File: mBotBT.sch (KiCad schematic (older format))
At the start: 6 parts, among them P101 CONN_01X04, P102 CONN_01X03, U101 LM1084IT-3.3/NOPB, U102 XBEE

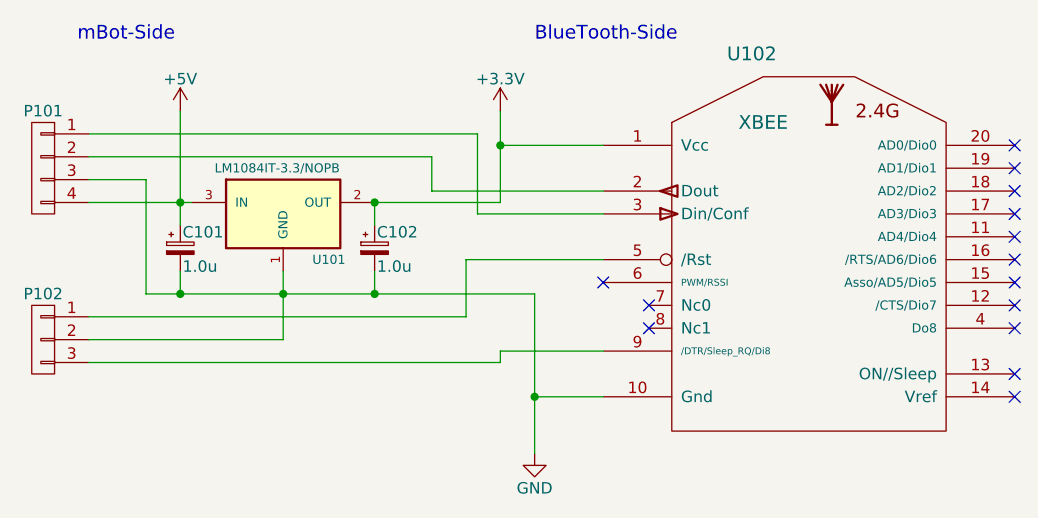
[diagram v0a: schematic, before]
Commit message: Bugfix
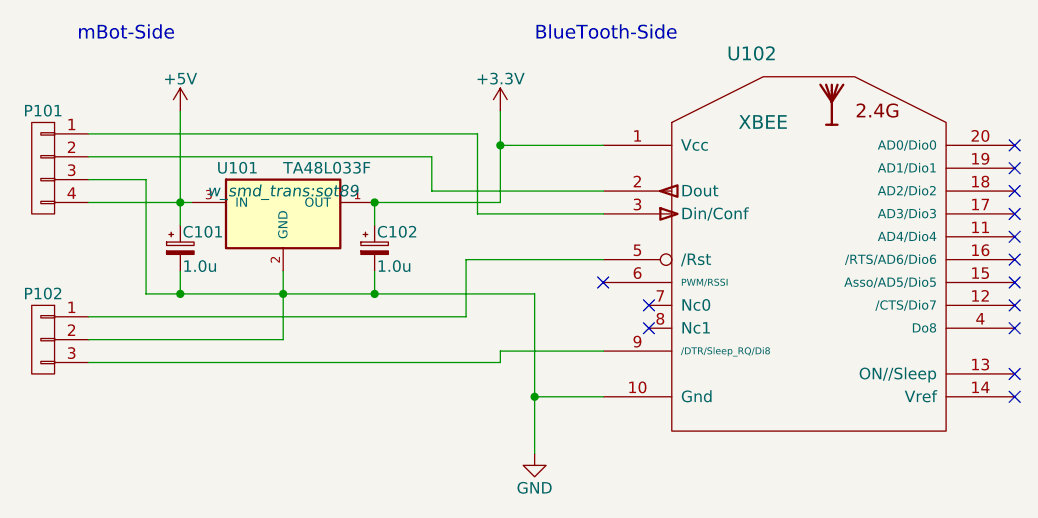
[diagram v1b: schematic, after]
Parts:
- removed U101: LM1084IT-3.3/NOPB, w_smd_trans:sot89, symbol LM1084IT-3.3/NOPB
- added U101: TA48L033F, w_smd_trans:sot89, symbol MC78L08ACH
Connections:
- net +3V3: now also U101.1 (OUT)
- net +5V: now also U101.3 (IN)
- net GND: now also U101.2 (GND)
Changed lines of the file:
@@
 BlueTooth-Side
-$Comp
-L LM1084IT-3.3/NOPB U101
-U 1 1 56B5416D
-P 4700 2500
-F 0 "U101" H 4900 2300 40  0000 C CNN
-F 1 "LM1084IT-3.3/NOPB" H 4400 2700 40  0000 L CNN
-F 2 "w_smd_trans:sot89" H 4700 2600 30  0001 C CIN
-F 3 "" H 4700 2500 60  0000 C CNN
-	1    4700 2500
-	1    0    0    -1
-$EndComp
 $Comp
 L CP_Small C101
@@
 	1    0    0    -1
 $EndComp
+NoConn ~ 6300 3000
+NoConn ~ 6300 2900
+NoConn ~ 6100 2800
+NoConn ~ 7900 2200
+NoConn ~ 7900 2300
+NoConn ~ 7900 2400
+NoConn ~ 7900 2500
+NoConn ~ 7900 2600
+NoConn ~ 7900 2700
+NoConn ~ 7900 2800
+NoConn ~ 7900 2900
+NoConn ~ 7900 3000
+NoConn ~ 7900 3200
+NoConn ~ 7900 3300
 Wire Wire Line
 	3850 2450 4300 2450
@@
 	5350 2250 3850 2250
 Wire Wire Line
-	5650 2450 5100 2450
-Wire Wire Line
-	5650 2050 5650 2450
+	5650 2450 5650 2050
 Wire Wire Line
 	5650 2200 6100 2200
@@
 Connection ~ 4700 2850
 Wire Wire Line
-	5100 2450 5100 2550
-Wire Wire Line
 	4250 2750 4250 2850
 Connection ~ 4250 2850
@@
 	4250 2050 4250 2550
 Connection ~ 4250 2450
-Connection ~ 5100 2450
 Wire Wire Line
 	4700 3050 3850 3050
@@
 Connection ~ 5650 2200
 Connection ~ 5800 3300
-NoConn ~ 6300 3000
-NoConn ~ 6300 2900
-NoConn ~ 6100 2800
-NoConn ~ 7900 2200
-NoConn ~ 7900 2300
-NoConn ~ 7900 2400
-NoConn ~ 7900 2500
-NoConn ~ 7900 2600
-NoConn ~ 7900 2700
-NoConn ~ 7900 2800
-NoConn ~ 7900 2900
-NoConn ~ 7900 3000
-NoConn ~ 7900 3200
-NoConn ~ 7900 3300
 Wire Wire Line
 	5650 3100 6100 3100
@@
 Wire Wire Line
 	4100 2350 4100 2850
+$Comp
+L MC78L08ACH U101
+U 1 1 56EE1811
+P 4700 2500
+F 0 "U101" H 4500 2700 50  0000 C CNN
+F 1 "TA48L033F" H 4700 2700 50  0000 L CNN
+F 2 "w_smd_trans:sot89" H 4700 2600 50  0000 C CIN
+F 3 "" H 4700 2500 50  0000 C CNN
+	1    4700 2500
+	1    0    0    -1
+$EndComp
+Wire Wire Line
+	5100 2450 5650 2450
+Wire Wire Line
+	5100 2550 5100 2450
+Connection ~ 5100 2450
 $EndSCHEMATC
